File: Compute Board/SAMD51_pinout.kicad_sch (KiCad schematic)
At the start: 10 parts, among them U11 SAMD51

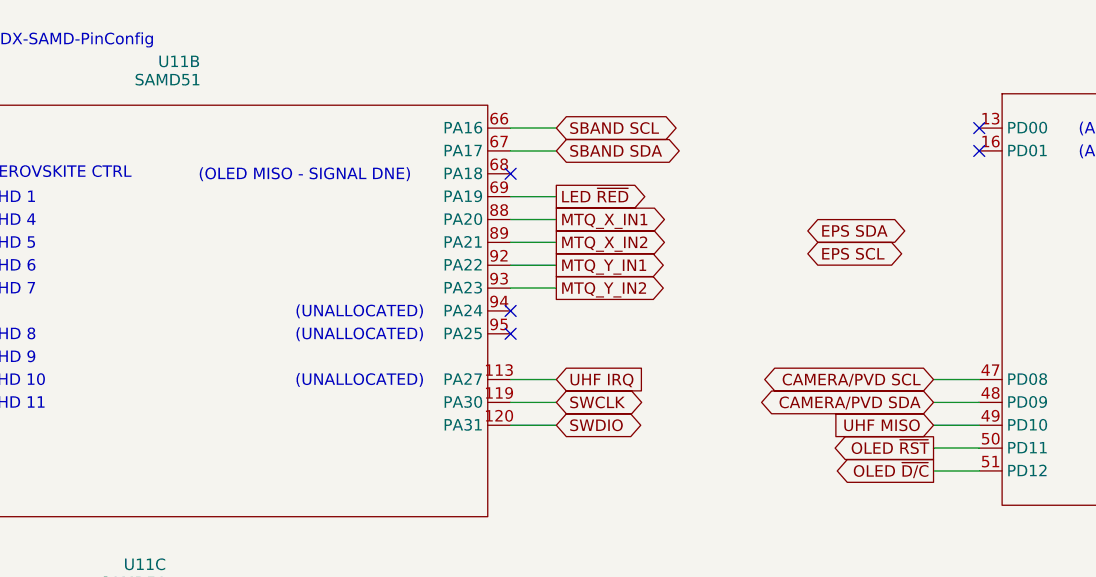
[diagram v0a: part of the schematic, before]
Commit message: Finished routing
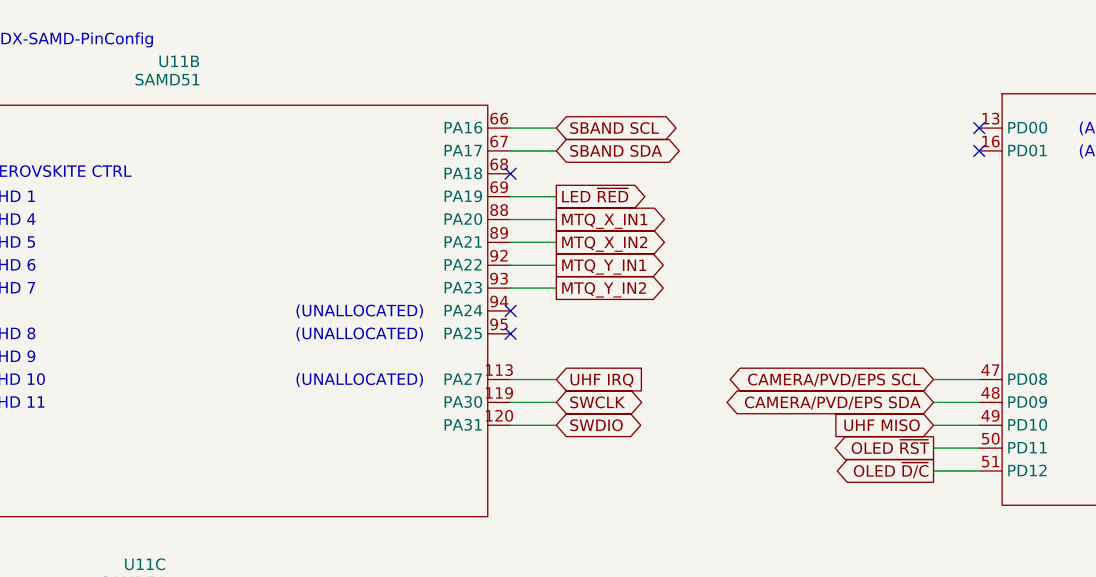
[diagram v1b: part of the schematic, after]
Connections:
- net CAMERA/PVD SCL renamed CAMERA/PVD/EPS SCL
- net CAMERA/PVD SDA renamed CAMERA/PVD/EPS SDA
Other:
- note removed: "(OLED MISO - SIGNAL DNE)"
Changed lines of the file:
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@@
 		)
 	)
-	(text "(OLED MISO - SIGNAL DNE)"
-		(exclude_from_sim no)
-		(at 101.6 37.084 0)
-		(effects
-			(font
-				(size 1.27 1.27)
-				(color 255 0 0 1)
-			)
-		)
-	)
 	(text "THERM 3"
 		(exclude_from_sim no)
@@
 		)
 	)
-	(global_label "EPS SDA"
+	(global_label "CAMERA{slash}PVD{slash}EPS SDA"
 		(shape bidirectional)
-		(at 157.48 43.18 0)
-		(fields_autoplaced yes)
+		(at 171.45 62.23 180)
 		(effects
 			(font
 				(size 1.27 1.27)
 			)
-			(justify left)
+			(justify right)
 		)
 		(property "Intersheetrefs" "${INTERSHEET_REFS}"
-			(at 168.6294 43.18 0)
+			(at 156.3938 60.198 0)
 			(hide yes)
 			(show_name no)
@@
 					(size 1.27 1.27)
 				)
-				(justify left)
+				(justify right)
 			)
 		)
@@
 		)
 	)
+	(global_label "CAMERA{slash}PVD{slash}EPS SCL"
+		(shape bidirectional)
+		(at 171.45 59.69 180)
+		(effects
+			(font
+				(size 1.27 1.27)
+			)
+			(justify right)
+		)
+		(property "Intersheetrefs" "${INTERSHEET_REFS}"
+			(at 156.3938 57.658 0)
+			(hide yes)
+			(show_name no)
+			(do_not_autoplace no)
+			(effects
+				(font
+					(size 1.27 1.27)
+				)
+				(justify right)
+			)
+		)
+	)
 	(global_label "SWCLK"
 		(shape bidirectional)
@@
 		)
 	)
-	(global_label "CAMERA{slash}PVD SCL"
-		(shape bidirectional)
-		(at 171.45 59.69 180)
-		(effects
-			(font
-				(size 1.27 1.27)
-			)
-			(justify right)
-		)
-		(property "Intersheetrefs" "${INTERSHEET_REFS}"
-			(at 156.3938 57.658 0)
-			(hide yes)
-			(show_name no)
-			(do_not_autoplace no)
-			(effects
-				(font
-					(size 1.27 1.27)
-				)
-				(justify right)
-			)
-		)
-	)
 	(global_label "ADC1 AIN9"
 		(shape input)
@@
 		)
 	)
-	(global_label "CAMERA{slash}PVD SDA"
-		(shape bidirectional)
-		(at 171.45 62.23 180)
-		(effects
-			(font
-				(size 1.27 1.27)
-			)
-			(justify right)
-		)
-		(property "Intersheetrefs" "${INTERSHEET_REFS}"
-			(at 156.3938 60.198 0)
-			(hide yes)
-			(show_name no)
-			(do_not_autoplace no)
-			(effects
-				(font
-					(size 1.27 1.27)
-				)
-				(justify right)
-			)
-		)
-	)
 	(global_label "MTQ_Y_IN2"
 		(shape output)
@@
 			(hide yes)
 			(show_name no)
-			(do_not_autoplace no)
-			(effects
-				(font
-					(size 1.27 1.27)
-				)
-				(justify left)
-			)
-		)
-	)
-	(global_label "EPS SCL"
-		(shape bidirectional)
-		(at 157.48 45.72 0)
-		(fields_autoplaced yes)
-		(effects
-			(font
-				(size 1.27 1.27)
-			)
-			(justify left)
-		)
-		(property "Intersheetrefs" "${INTERSHEET_REFS}"
-			(at 168.5689 45.72 0)
-			(hide yes)
-			(show_name no)
